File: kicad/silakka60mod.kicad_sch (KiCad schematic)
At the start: 63 parts, among them J1 AudioJack4, J2 AudioJack4, U1 RP2040_Zero

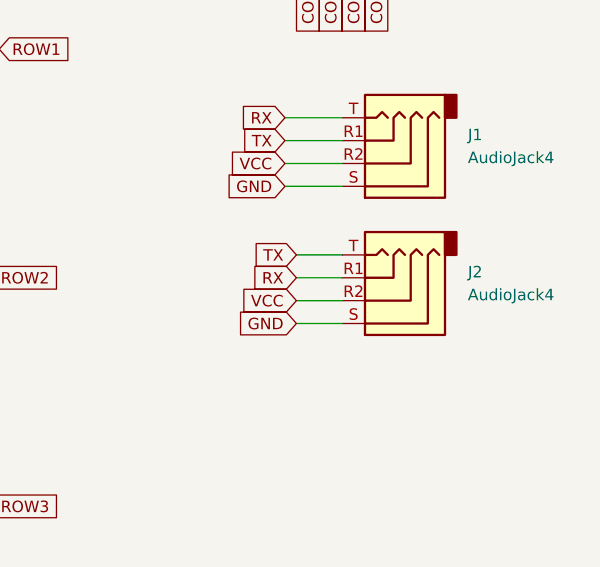
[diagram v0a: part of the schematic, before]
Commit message: Add files via upload
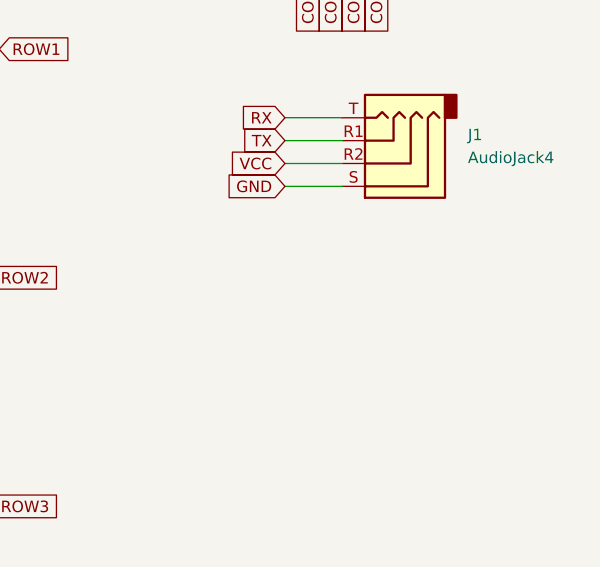
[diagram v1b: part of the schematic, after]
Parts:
- removed J2: AudioJack4, Connector_Audio:Jack_3.5mm_PJ320D_Horizontal, symbol Connector_Audio:AudioJack4
- D1, D10, D11, D12, D13, D14, D15, D16, D17, D18, D19, D2, D20, D21, D22, D23, D24, D25, D26, D27, D28, D29, D3, D30, D4, D5, D6, D7, D8, D9: footprint ScottoKeebs_Components:Diode_DO-35 -> SCOTTOKEEBS components:Diode_DO-35
- S1, S10, S11, S12, S13, S14, S15, S16, S17, S18, S19, S2, S20, S21, S22, S23, S24, S25, S26, S27, S28, S29, S3, S30, S4, S5, S6, S7, S8, S9: footprint kbd:CherryMX_MidHeight_Hotswap -> kbd:keyswitch_cherrymx_hotswap_1u
- U1: footprint ScottoKeebs_MCU:RP2040_Zero -> SCOTTOKEEBS mcu:RP2040_Zero
